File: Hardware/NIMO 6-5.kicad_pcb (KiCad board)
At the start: 2 copper layers, 249.9 x 140.4 mm, 66 parts, among them J1 M1, J2 Screw_Terminal_01x04, J5 QTR8A, SW1 SW_SPDT_321, SW2 SW_PUSH, U1 ESP32-DEVKITC-32D, U2 TB6612_BREAKOUT, U3 L7805

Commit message: cambio de placa
.......
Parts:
- removed the C1 at (217.0, 95.1)
- removed the C1 at (125.1, 94.8)
- removed the C1 at (33.0, 95.0)
- removed the C2 at (33.0, 102.7)
- removed the C2 at (217.0, 102.8)
- removed the C2 at (125.1, 102.4)
- removed the C3 at (145.1, 107.5)
- removed the C3 at (53.0, 107.7)
- removed the C3 at (237.0, 107.9)
- removed C5 (x3): C, Capacitor_THT:C_Disc_D3.8mm_W2.6mm_P2.50mm
- removed the D1 at (38.4, 54.9)
- removed the D1 at (222.4, 55.1)
- removed the D1 at (130.5, 54.7)
- removed the D2 at (158.7, 94.2)
- removed the D2 at (250.6, 94.6)
- removed the D2 at (66.7, 94.4)
- removed the H1 at (157.4, 40.6)
- removed the H1 at (65.3, 40.8)
- removed the H1 at (249.3, 41.0)
- removed the H2 at (117.4, 149.6)
- removed the H2 at (25.3, 149.8)
- removed the H2 at (209.2, 149.9)
- removed the H3 at (250.9, 138.2)
- removed the H3 at (67.0, 138.1)
- removed the H3 at (159.0, 137.8)
- removed the H4 at (222.9, 138.2)
- removed the H4 at (38.9, 138.1)
- removed the H4 at (131.0, 137.8)
- removed the H5 at (224.6, 41.0)
- removed the H5 at (132.7, 40.6)
- removed the H5 at (40.6, 40.8)
- removed the H6 at (171.4, 149.6)
- removed the H6 at (263.3, 149.9)
- removed the H6 at (79.3, 149.8)
- removed the J1 at (139.0, 116.0)
- removed the J1 at (46.9, 116.2)
- removed the J1 at (230.8, 116.3)
- removed J2 (x3): Screw_Terminal_01x04, TerminalBlock:TerminalBlock_Altech_AK300-4_P5.00mm
- removed the J5 at (38.1, 46.7)
- removed the J5 at (130.2, 46.4)
- removed the J5 at (222.1, 46.8)
- removed the R1 at (215.4, 55.1)
- removed the R1 at (123.5, 54.7)
- removed the R1 at (31.4, 54.9)
- removed the R2 at (159.7, 85.6)
- removed the R2 at (251.6, 86.0)
- removed the R2 at (67.7, 85.8)
- removed the SW1 at (257.2, 101.2)
- removed the SW1 at (73.2, 101.0)
- removed the SW1 at (165.3, 100.8)
- removed the SW2 at (79.8, 94.4)
- removed the SW2 at (171.9, 94.2)
- removed the SW2 at (263.8, 94.6)
- removed the U1 at (146.1, 72.1)
- removed the U1 at (54.0, 72.3)
- removed the U1 at (238.0, 72.4)
- removed the U2 at (236.2, 93.5)
- removed the U2 at (144.3, 93.2)
- removed the U2 at (52.2, 93.4)
- removed the U3 at (27.1, 101.2)
- removed the U3 at (119.2, 101.0)
- removed the U3 at (211.1, 101.3)
- added C1: 10 u x 25, Capacitor_SMD:CP_Elec_8x6.2, F.Cu at (136.7, 120.4)
- added C2: 100 u x 25, Capacitor_SMD:CP_Elec_6.3x5.4, F.Cu at (136.7, 131.8)
- added C3: C, Capacitor_SMD:C_0805_2012Metric, B.Cu at (156.6, 140.3)
- added C4: C, Capacitor_SMD:C_0805_2012Metric, B.Cu at (161.7, 140.3)
- added D1: LED, LED_SMD:LED_0805_2012Metric, F.Cu at (122.9, 116.5)
- added D2: LED, LED_SMD:LED_0805_2012Metric, F.Cu at (189.7, 115.8)
- added H1: MountingHole, MountingHole:MountingHole_3.2mm_M3, F.Cu at (201.7, 131.0)
- added H2: MountingHole, MountingHole:MountingHole_3.2mm_M3, F.Cu at (110.1, 131.0)
- added H3: MountingHole, a:Pololu_Micro_Bracket_Wheel_42mms, F.Cu at (176.6, 152.4)
- added H4: MountingHole, a:Pololu_Micro_Bracket_Wheel_42mms, F.Cu at (137.4, 154.9)
- added H5: MountingHole, MountingHole:MountingHole_3.2mm_M3, F.Cu at (194.6, 94.1)
- added H6: MountingHole, MountingHole:MountingHole_3.2mm_M3, F.Cu at (119.5, 94.1)
- added J1: M1, Connector_PinHeader_2.54mm:PinHeader_1x02_P2.54mm_Vertical, F.Cu at (155.7, 144.5)
- added J3: M1, Connector_PinHeader_2.54mm:PinHeader_1x02_P2.54mm_Vertical, F.Cu at (162.7, 144.5)
- added J4: M1, TerminalBlock:TerminalBlock_Altech_AK300-2_P5.00mm, F.Cu at (187.8, 132.4)
- added J5: QTR8A, Connector_PinHeader_2.54mm:PinHeader_1x11_P2.54mm_Vertical, F.Cu at (144.2, 79.4)
- added R1: 1K, Resistor_SMD:R_0805_2012Metric_Pad1.20x1.40mm_HandSolder, F.Cu at (127.3, 116.5)
- added R2: 1K, Resistor_SMD:R_0805_2012Metric_Pad1.20x1.40mm_HandSolder, F.Cu at (185.3, 115.8)
- added SW1: SW_SPDT_321, a:SW_SPDT_TH_Vertical, F.Cu at (175.6, 127.4)
- added SW2: SW_PUSH, Button_Switch_THT:SW_PUSH_6mm_H5mm, F.Cu at (194.1, 108.4)
- added U1: ESP32-DEVKITC-32D, Library:MODULE_ESP32-DEVKITC-32D, F.Cu at (158.2, 104.4)
- added U2: TB6612_BREAKOUT, a:TB6612_Breakout, F.Cu at (156.6, 126.7)
- added U3: L7805, Package_TO_SOT_SMD:TO-263-2, F.Cu at (120.7, 126.3)
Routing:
- net VCC: track 317.7 -> 88.5 mm, vias 0 -> 1
- net +5V: track 328.7 -> 125.2 mm, vias 0 -> 1
- net Net-(J2-Pin_4): track 45.6 -> 0.00 mm
- net /B2: track 59.5 -> 14.7 mm
- net /B1: track 53.9 -> 10.3 mm
- net /A1: track 50.5 -> 10.3 mm
- net /s3: track 55.0 -> 15.8 mm
- net /s5: track 51.6 -> 15.8 mm
- net /s2: track 51.6 -> 15.8 mm
- net /s4: track 51.6 -> 15.8 mm
- net /s1: track 51.6 -> 15.8 mm
- net /s6: track 51.6 -> 15.9 mm
- net /s7: track 51.6 -> 16.8 mm
- net /s8: track 51.6 -> 17.3 mm
- net /A2: track 47.4 -> 14.7 mm
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- added copper zone on F.Cu, net GND
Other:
- board size 249.9 x 140.4 mm -> 140 x 120.1 mm

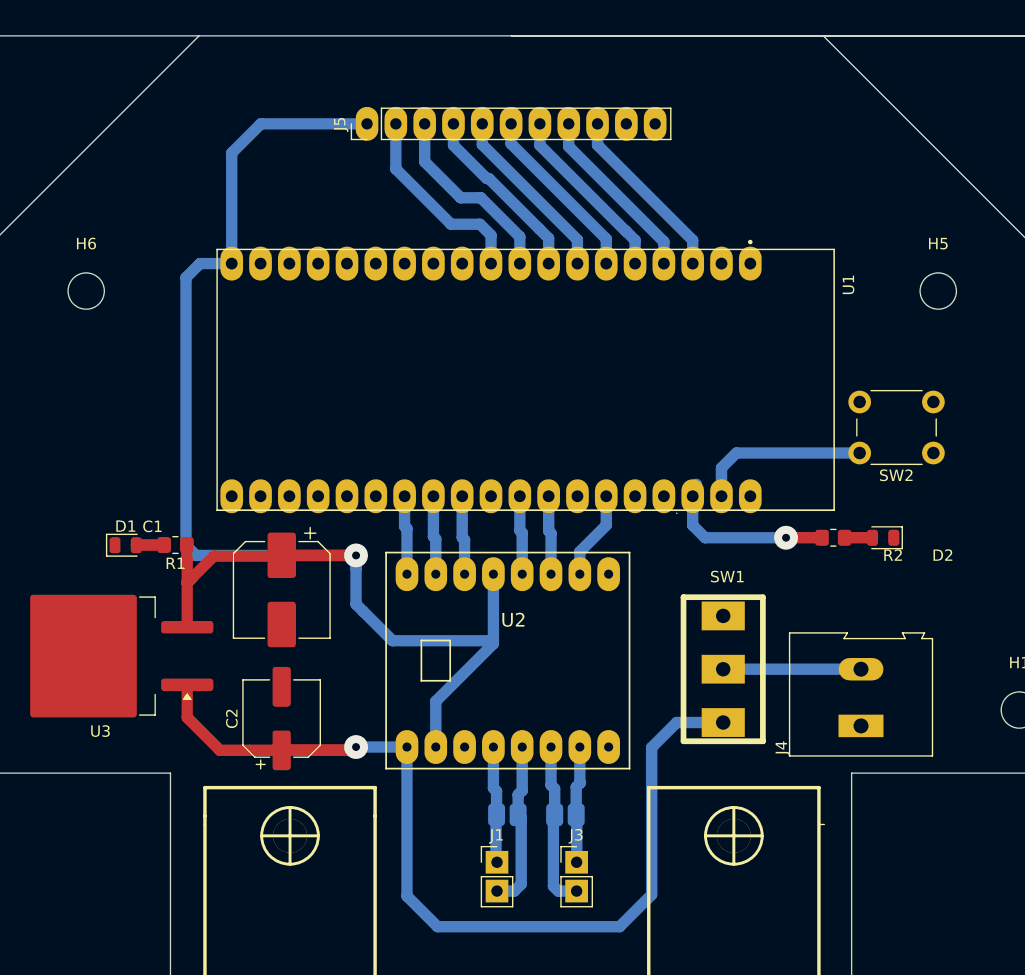
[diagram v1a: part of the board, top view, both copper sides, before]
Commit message: cambio de placa
12/5/26
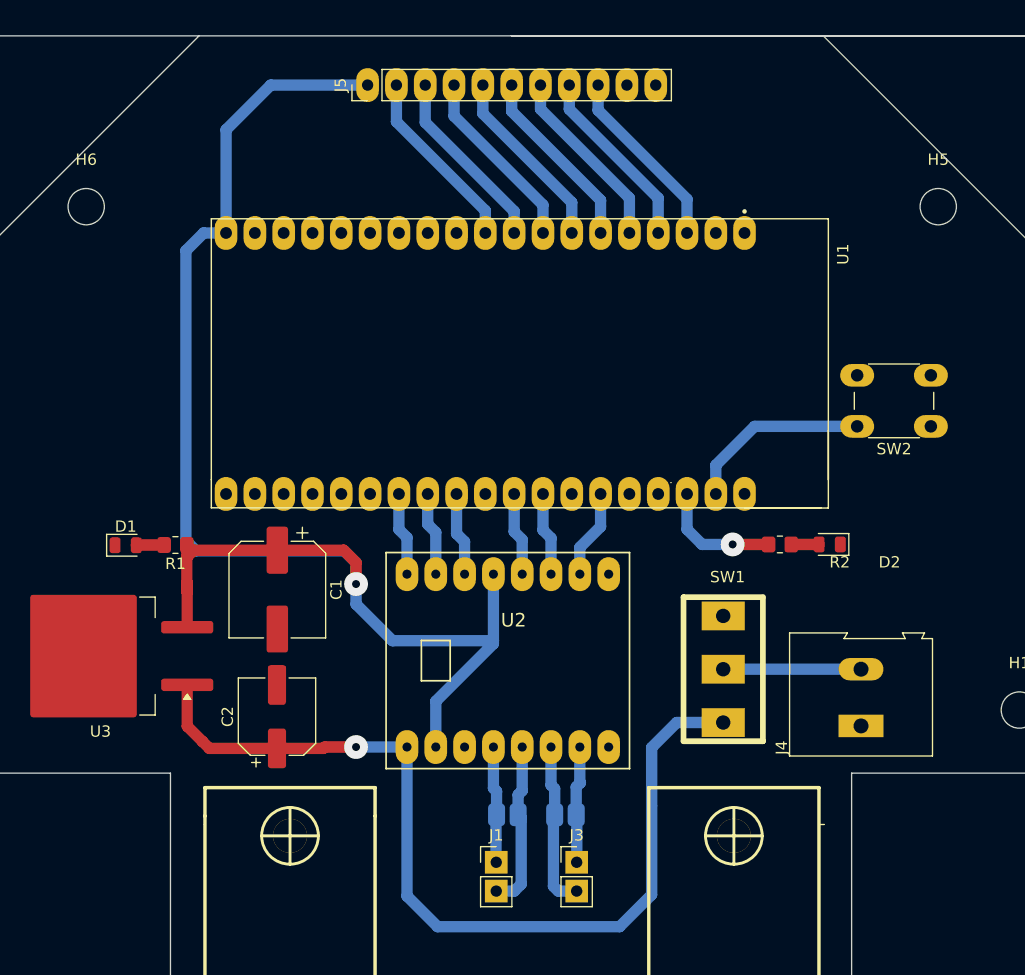
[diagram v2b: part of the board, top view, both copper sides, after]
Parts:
- C1: footprint Capacitor_SMD:CP_Elec_8x6.2 -> Capacitor_SMD:CP_Elec_8x6.9
- C2: footprint Capacitor_SMD:CP_Elec_6.3x5.4 -> Capacitor_SMD:CP_Elec_6.3x5.9
- moved H5 7.44 mm to (194.6, 86.7)
- moved H6 7.44 mm to (119.5, 86.7)
- moved D2 4.75 mm to (185.0, 116.4)
- moved R2 4.75 mm to (180.6, 116.4)
- moved J5 3.42 mm to (144.3, 75.9)
- moved U1 2.75 mm to (157.7, 101.7)
- moved SW2 2.36 mm to (193.9, 106.0)
- moved C2 0.44 mm to (136.3, 131.6)
- moved C1 0.39 mm to (136.3, 120.4)
- moved J1 0.07 mm to (155.6, 144.5)
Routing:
- net VCC: track 88.5 -> 82.7 mm
- net /R: track 15.7 -> 10.9 mm
- net +5V: track 125.2 -> 128.9 mm
- net /SW: track 15.2 -> 16.4 mm
- net /s8: track 17.3 -> 16.3 mm
- net /s7: track 16.8 -> 16.3 mm

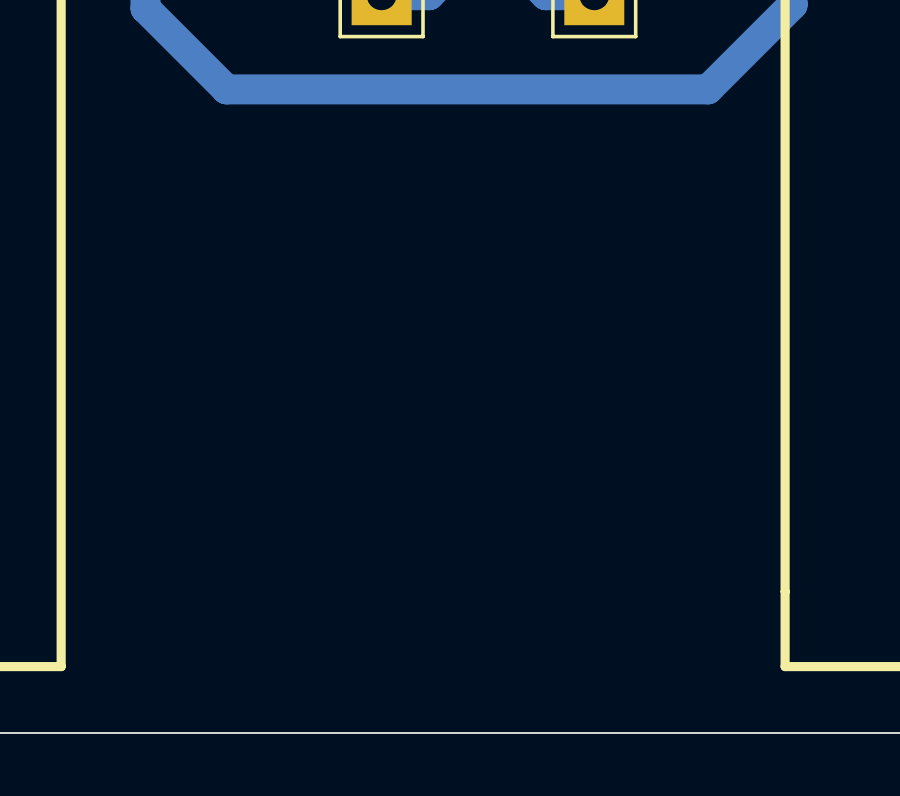
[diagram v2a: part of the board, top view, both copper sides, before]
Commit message: logo de la escuela
12/5/26-13:36
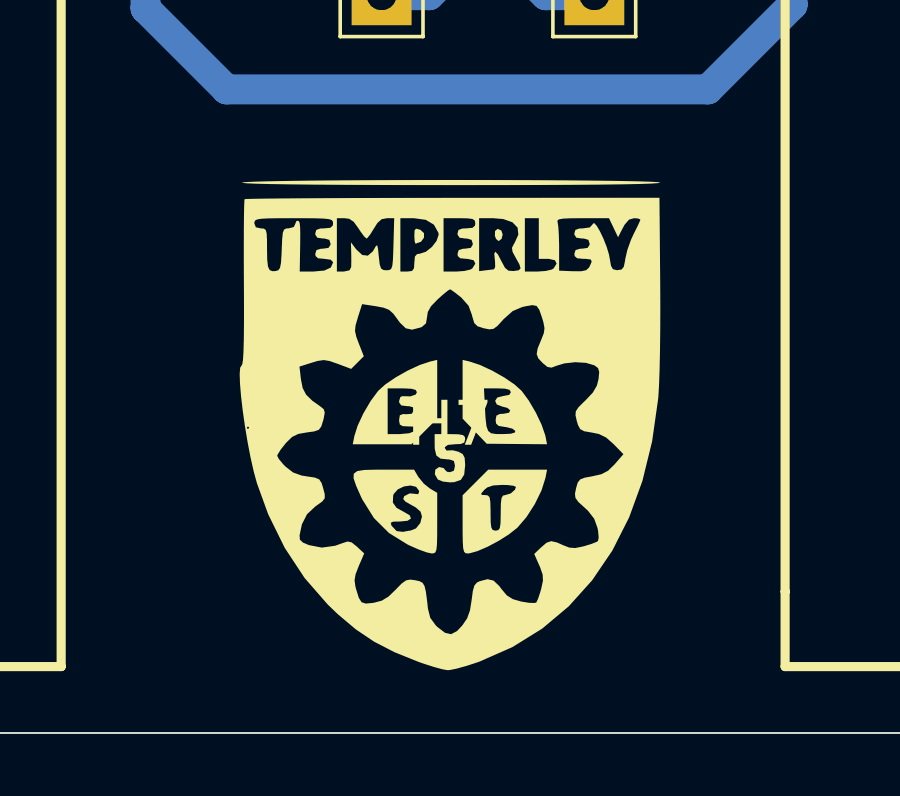
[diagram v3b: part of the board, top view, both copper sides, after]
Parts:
- added H7: MountingHole, a:school, F.Cu at (157.9, 161.3)
